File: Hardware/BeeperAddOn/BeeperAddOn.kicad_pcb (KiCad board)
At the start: 2 copper layers, 12.8 x 20.1 mm, 6 parts, among them J1 Conn_01x03_Socket, Q1 BSS138

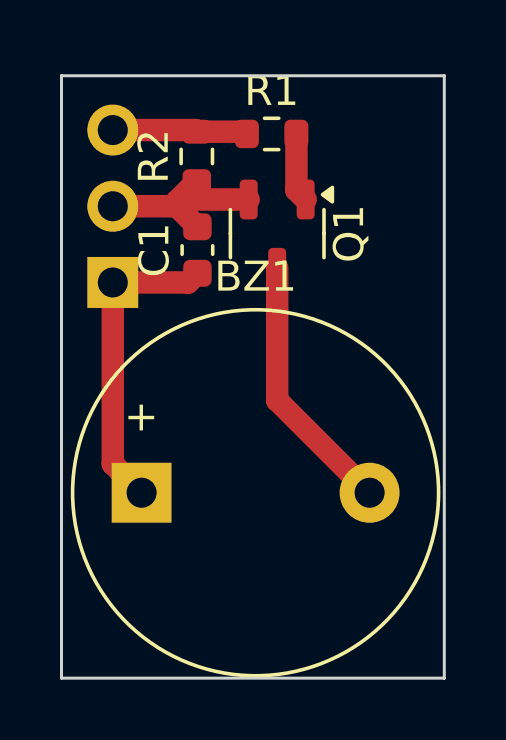
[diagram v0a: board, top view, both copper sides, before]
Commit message: buzzer
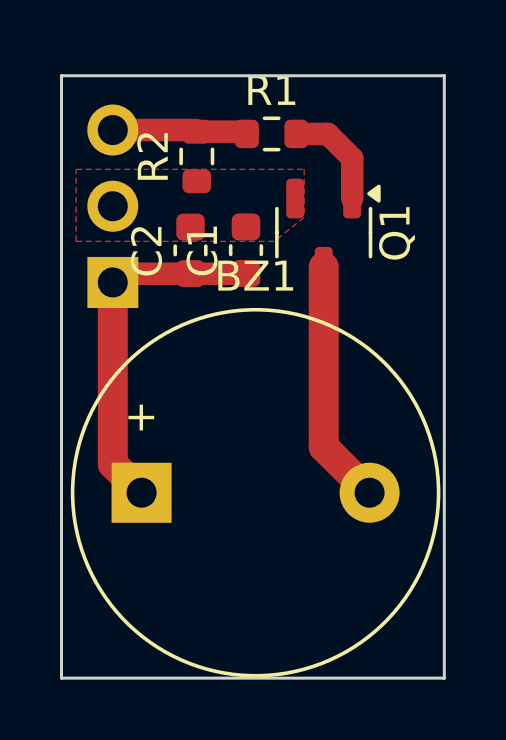
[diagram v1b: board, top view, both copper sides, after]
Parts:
- added C2: C, Capacitor_SMD:C_0603_1608Metric, F.Cu at (147.7, 106.2)
- moved C1 1.62 mm to (149.6, 106.2)
- moved Q1 1.55 mm to (152.2, 105.6)
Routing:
- net GND: track 6.70 -> 0.00 mm
- net +3.3V: track 10.4 -> 12.0 mm
- net Net-(Q1-G): track 2.31 -> 3.54 mm
- net Net-(BZ1--): track 8.78 -> 8.17 mm
- added copper zone on F.Cu, net GND
